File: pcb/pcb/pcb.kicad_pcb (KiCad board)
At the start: 2 copper layers, 58.4 x 44.4 mm, 26 parts, among them J1 UART, J2 Barrel_Jack, J3 Stepper, SW1 RESET, SW2 FLASH, U1 ESP32-WROOM-32, U2 TSR_1-2433

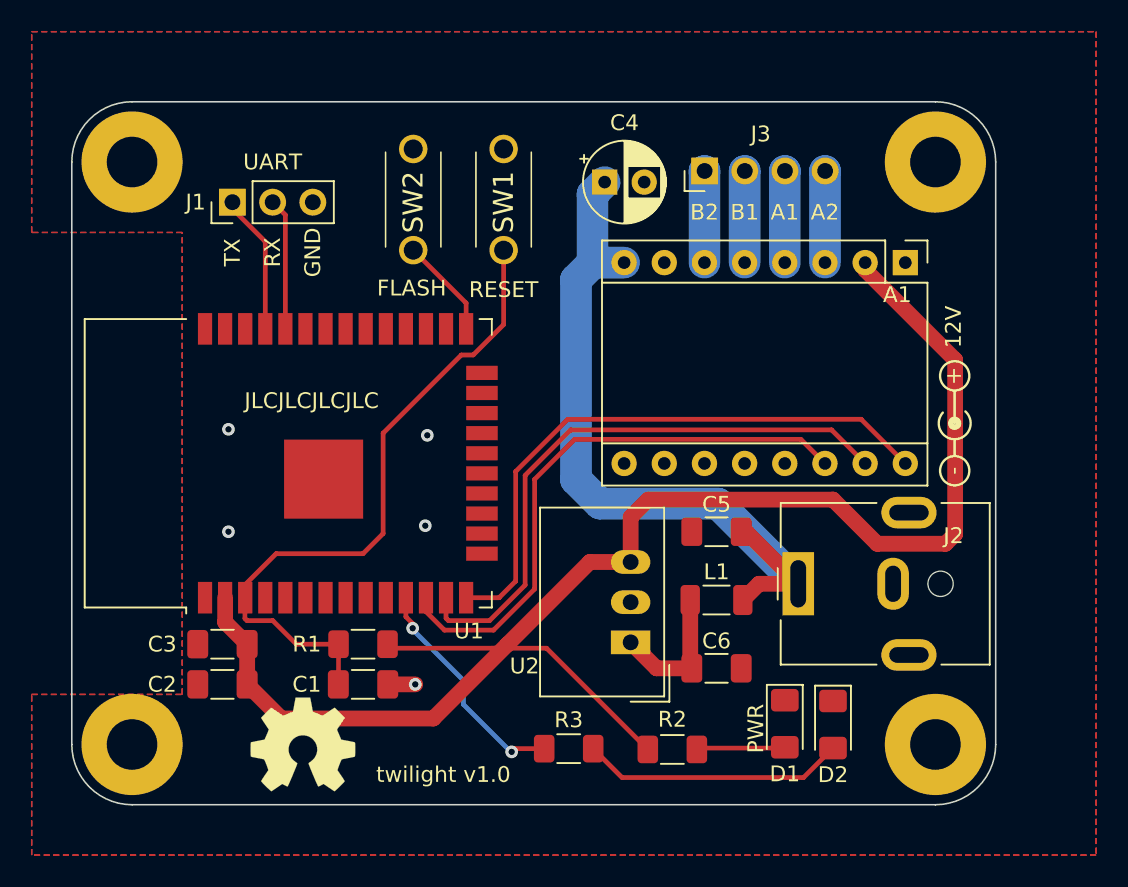
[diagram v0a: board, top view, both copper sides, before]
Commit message: third reddit revision
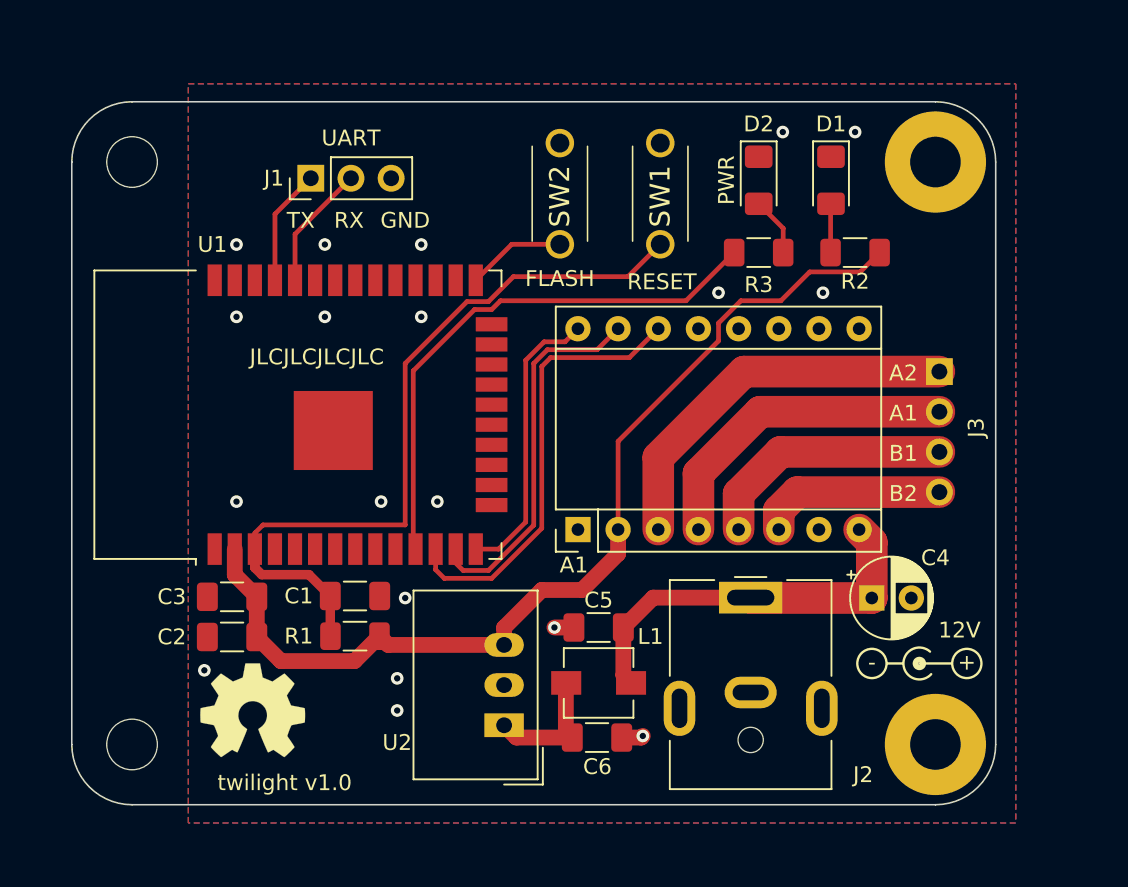
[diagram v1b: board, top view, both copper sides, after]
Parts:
- H1, H3: footprint MountingHole:MountingHole_3.2mm_M3_Pad -> MountingHole:MountingHole_3.2mm_M3
- L1: footprint Inductor_SMD:L_1206_3216Metric_Pad1.22x1.90mm_HandSolder -> Inductor_SMD:L_TracoPower_TCK-141
- moved D2 34.7 mm to (120.9, 48.8)
- moved D1 34.5 mm to (125.5, 48.8)
- moved R3 33.6 mm to (120.9, 53.3)
- moved R2 33.5 mm to (127.0, 53.3), turned to 180 degrees
- moved C4 31.3 mm to (128.1, 75.2)
- moved A1 26.7 mm to (109.5, 70.9), turned to 90 degrees
- moved J3 19.5 mm to (132.3, 60.9), turned to 0 degrees
- moved REF** 15.3 mm to (131.1, 79.2), turned to 0 degrees
- moved SW1 9.91 mm to (114.7, 52.8)
- moved C5 9.60 mm to (110.8, 77.0)
- moved U2 9.57 mm to (104.8, 83.2)
- moved SW2 9.28 mm to (108.3, 52.8)
- moved L1 9.11 mm to (110.8, 80.6)
- moved C6 8.73 mm to (110.7, 84.0)
- moved C1 5.61 mm to (95.4, 75.1)
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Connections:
- J3 pad 1: /B2 -> /A2
- J3 pad 2: /B1 -> /A1
- J3 pad 3: /A1 -> /B1
- J3 pad 4: /A2 -> /B2
- U1 pad 39: GND -> (no net)
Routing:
- net +3V3: track 99.9 -> 62.8 mm
- net +12V: track 47.3 -> 24.9 mm
- net Net-(R3-Pad1): track 14.7 -> 34.7 mm, vias 2 -> 0
- net /DIR: track 37.7 -> 18.2 mm
- net /A2: track 5.80 -> 24.6 mm
- net /A1: track 5.80 -> 20.4 mm
- net /STEP: track 37.8 -> 23.7 mm
- net Net-(D2-Pad2): track 16.7 -> 3.73 mm
- net /B1: track 5.80 -> 16.1 mm
- net /SLP: track 36.3 -> 28.1 mm
- net /EN: track 42.0 -> 49.4 mm
- net /B2: track 5.80 -> 11.8 mm
- net Net-(D1-Pad2): track 5.98 -> 3.10 mm
- net /TX: track 8.45 -> 7.39 mm
- net GND: track 1.74 -> 2.61 mm, vias 5 -> 19
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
